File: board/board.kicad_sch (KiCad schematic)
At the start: 38 parts, among them U101 Pico, U102 CS42438

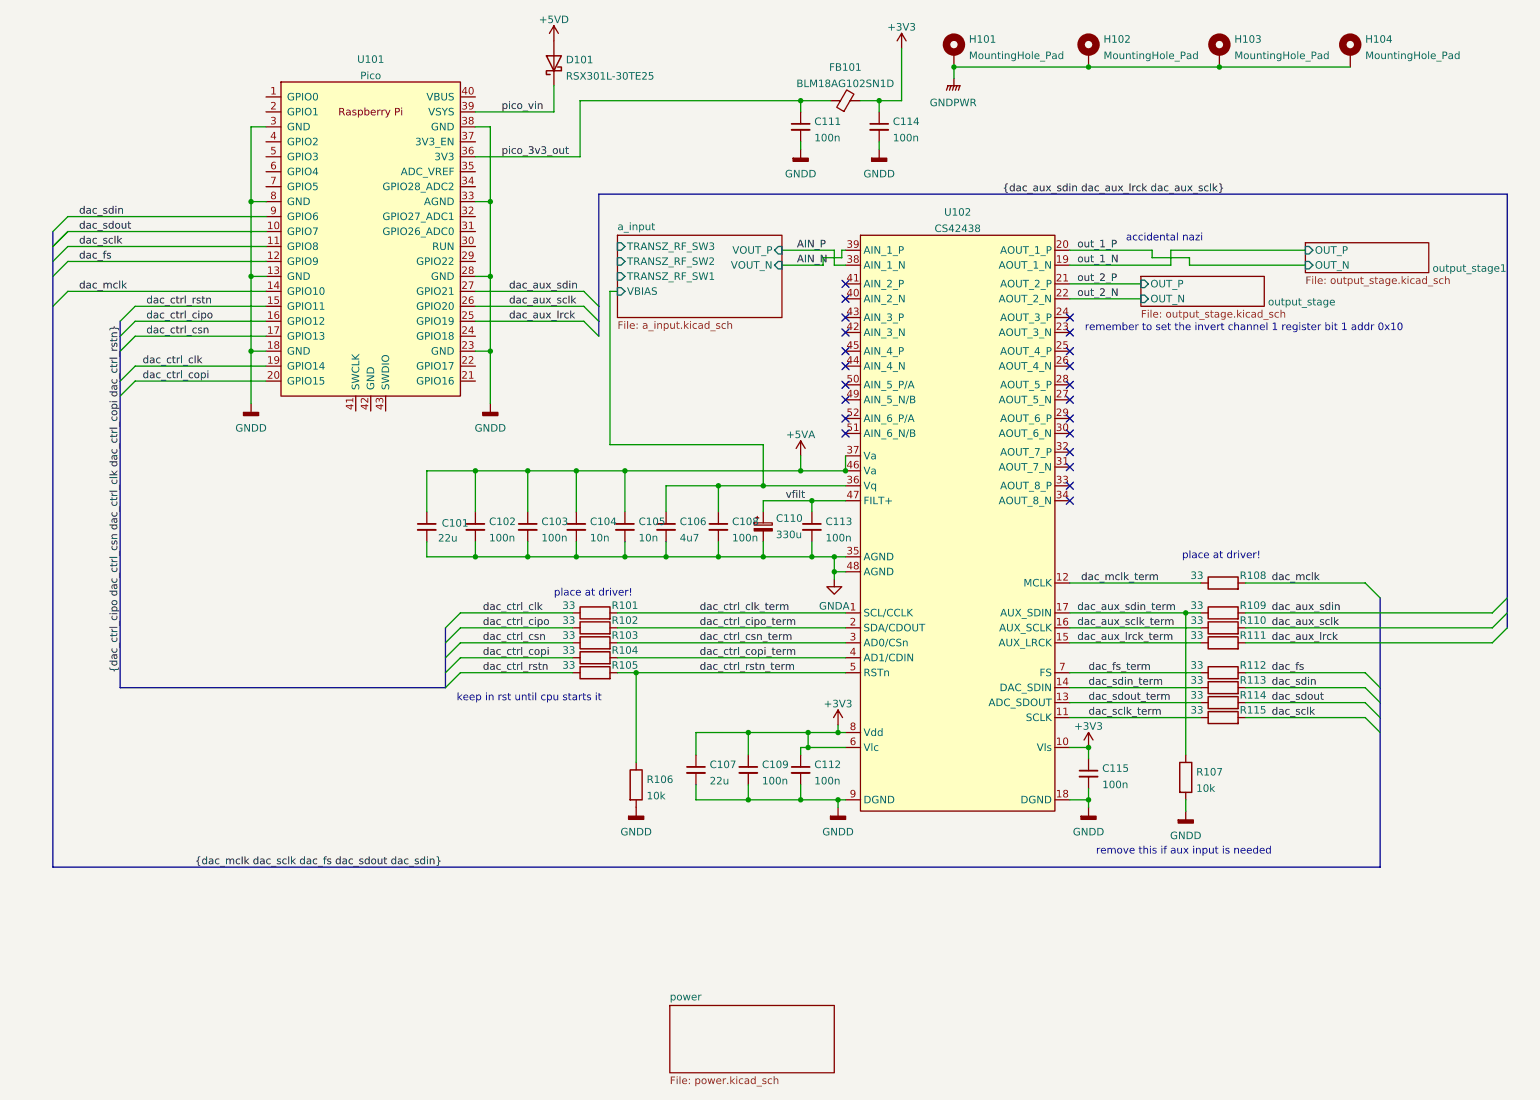
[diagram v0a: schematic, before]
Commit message: pcb done
attempt at doing some sw. builds but not tested
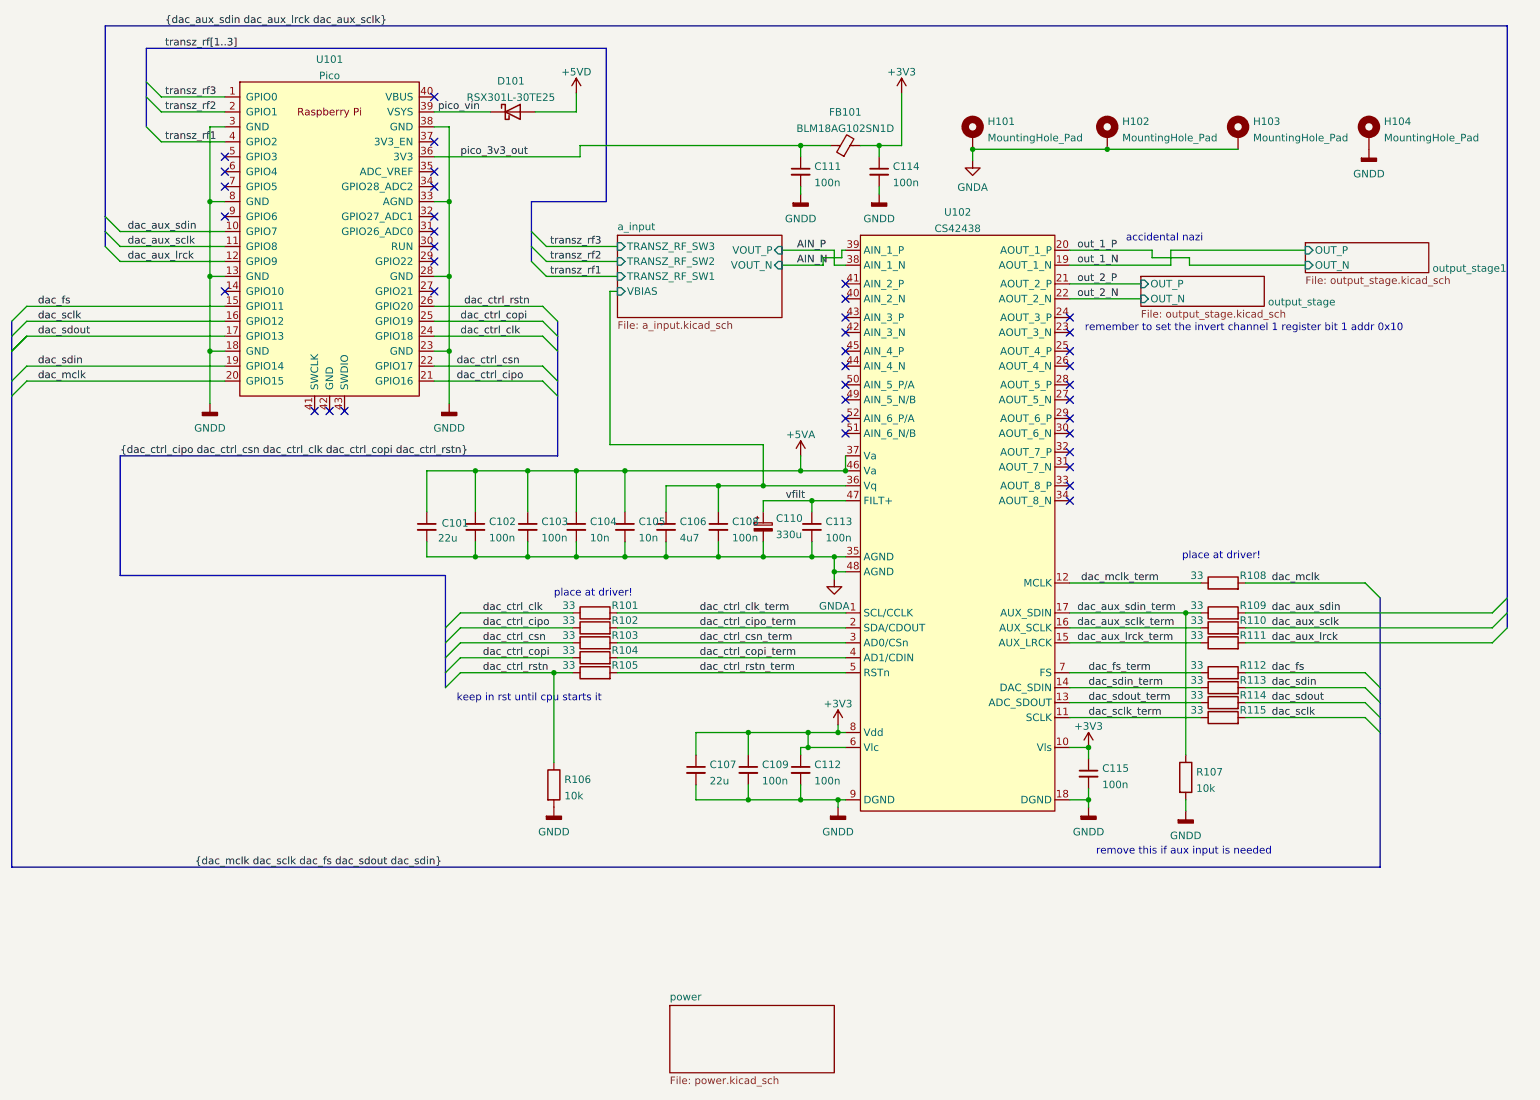
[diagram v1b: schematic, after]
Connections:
- net GNDA: now also H101.1, H102.1, H103.1
- net GNDD: now also H104.1
- net dac_aux_lrck: now also U101.12 (GPIO9); no longer U101.25 (GPIO19)
- net dac_aux_sclk: now also U101.11 (GPIO8); no longer U101.26 (GPIO20)
- net dac_aux_sdin: now also U101.10 (GPIO7); no longer U101.27 (GPIO21)
- net dac_ctrl_cipo: now also U101.21 (GPIO16); no longer U101.16 (GPIO12)
- net dac_ctrl_clk: now also U101.24 (GPIO18); no longer U101.19 (GPIO14)
- net dac_ctrl_copi: now also U101.25 (GPIO19); no longer U101.20 (GPIO15)
- net dac_ctrl_csn: now also U101.22 (GPIO17); no longer U101.17 (GPIO13)
- net dac_ctrl_rstn: now also R106.1, U101.26 (GPIO20); no longer U101.15 (GPIO11)
- net dac_ctrl_rstn_term: no longer R106.1
- net dac_fs: now also U101.15 (GPIO11); no longer U101.12 (GPIO9)
- net dac_mclk: now also U101.20 (GPIO15); no longer U101.14 (GPIO10)
- net dac_sclk: now also U101.16 (GPIO12); no longer U101.11 (GPIO8)
- net dac_sdin: now also U101.19 (GPIO14); no longer U101.9 (GPIO6)
- net dac_sdout: now also U101.17 (GPIO13); no longer U101.10 (GPIO7)
- net transz_rf3: now reaches U101.1 (GPIO0)
- net transz_rf2: now reaches U101.2 (GPIO1)
- net transz_rf1: now reaches U101.4 (GPIO2)
- removed net GNDPWR: H101.1, H102.1, H103.1, H104.1
- no-connect marks 22 -> 39
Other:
- moved on the sheet: C111, C114, D101, FB101, H101, H102, H103, H104, R106, U101
